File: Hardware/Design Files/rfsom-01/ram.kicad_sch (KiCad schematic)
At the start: 32 parts

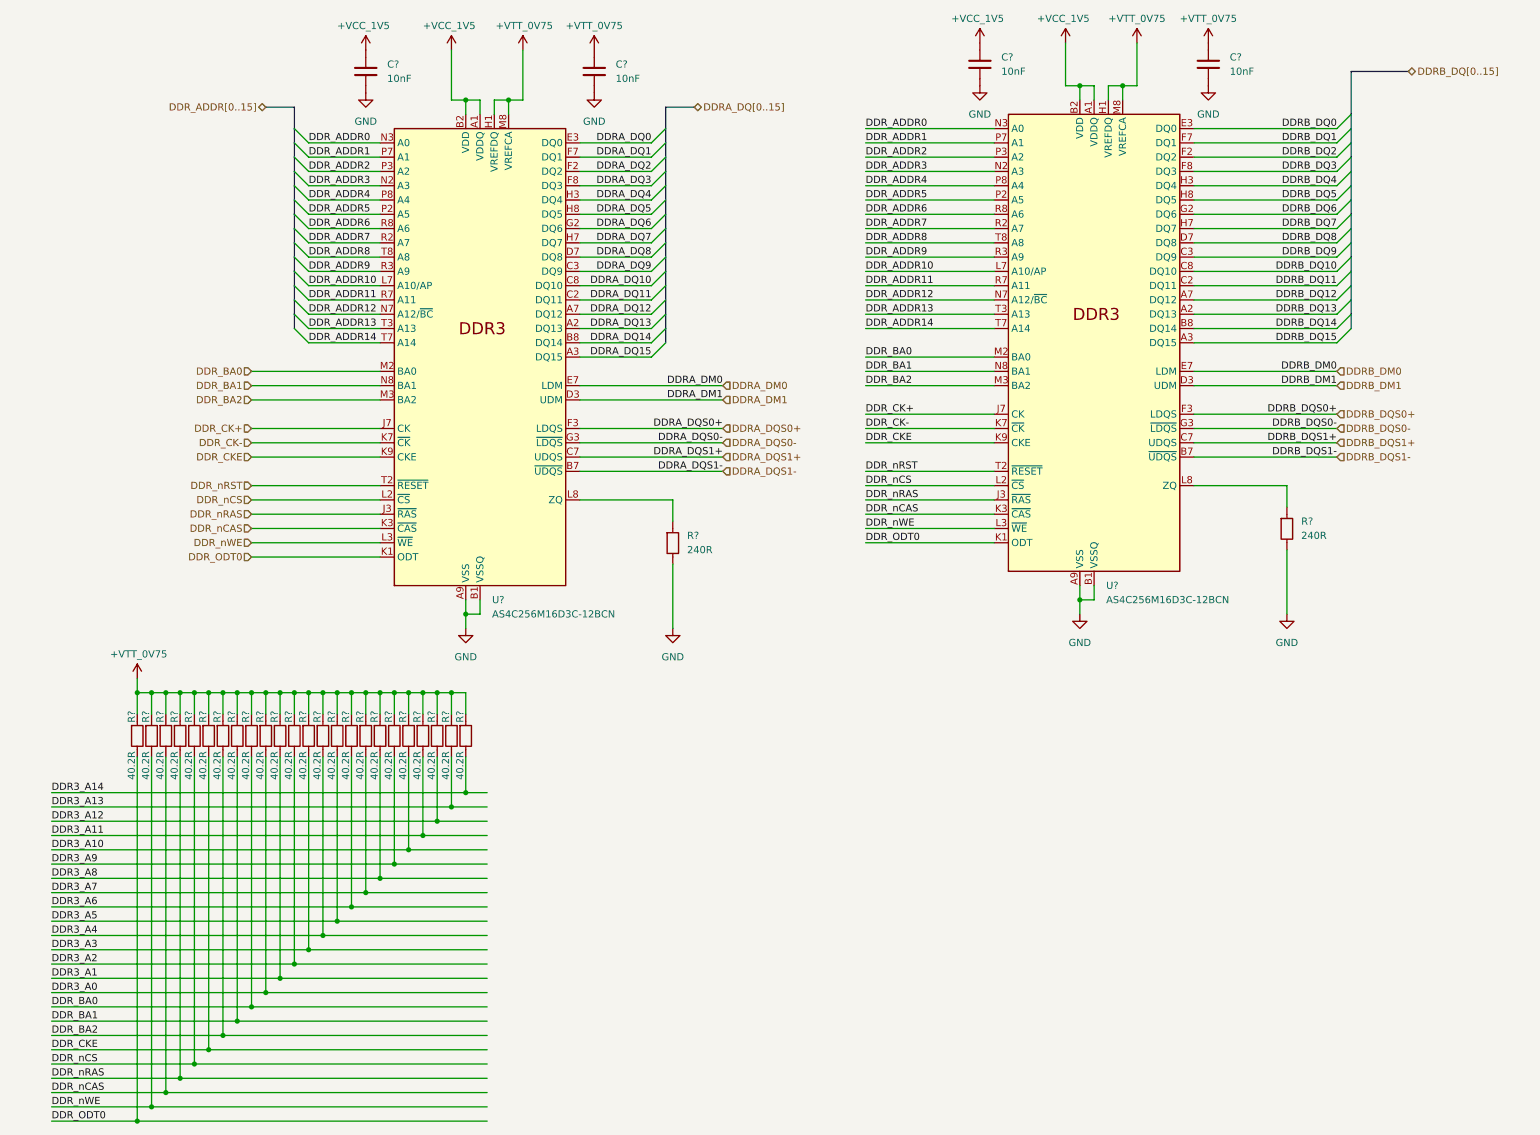
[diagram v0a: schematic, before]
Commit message: ps progress; added ftdi; mezz pinout pedinging;
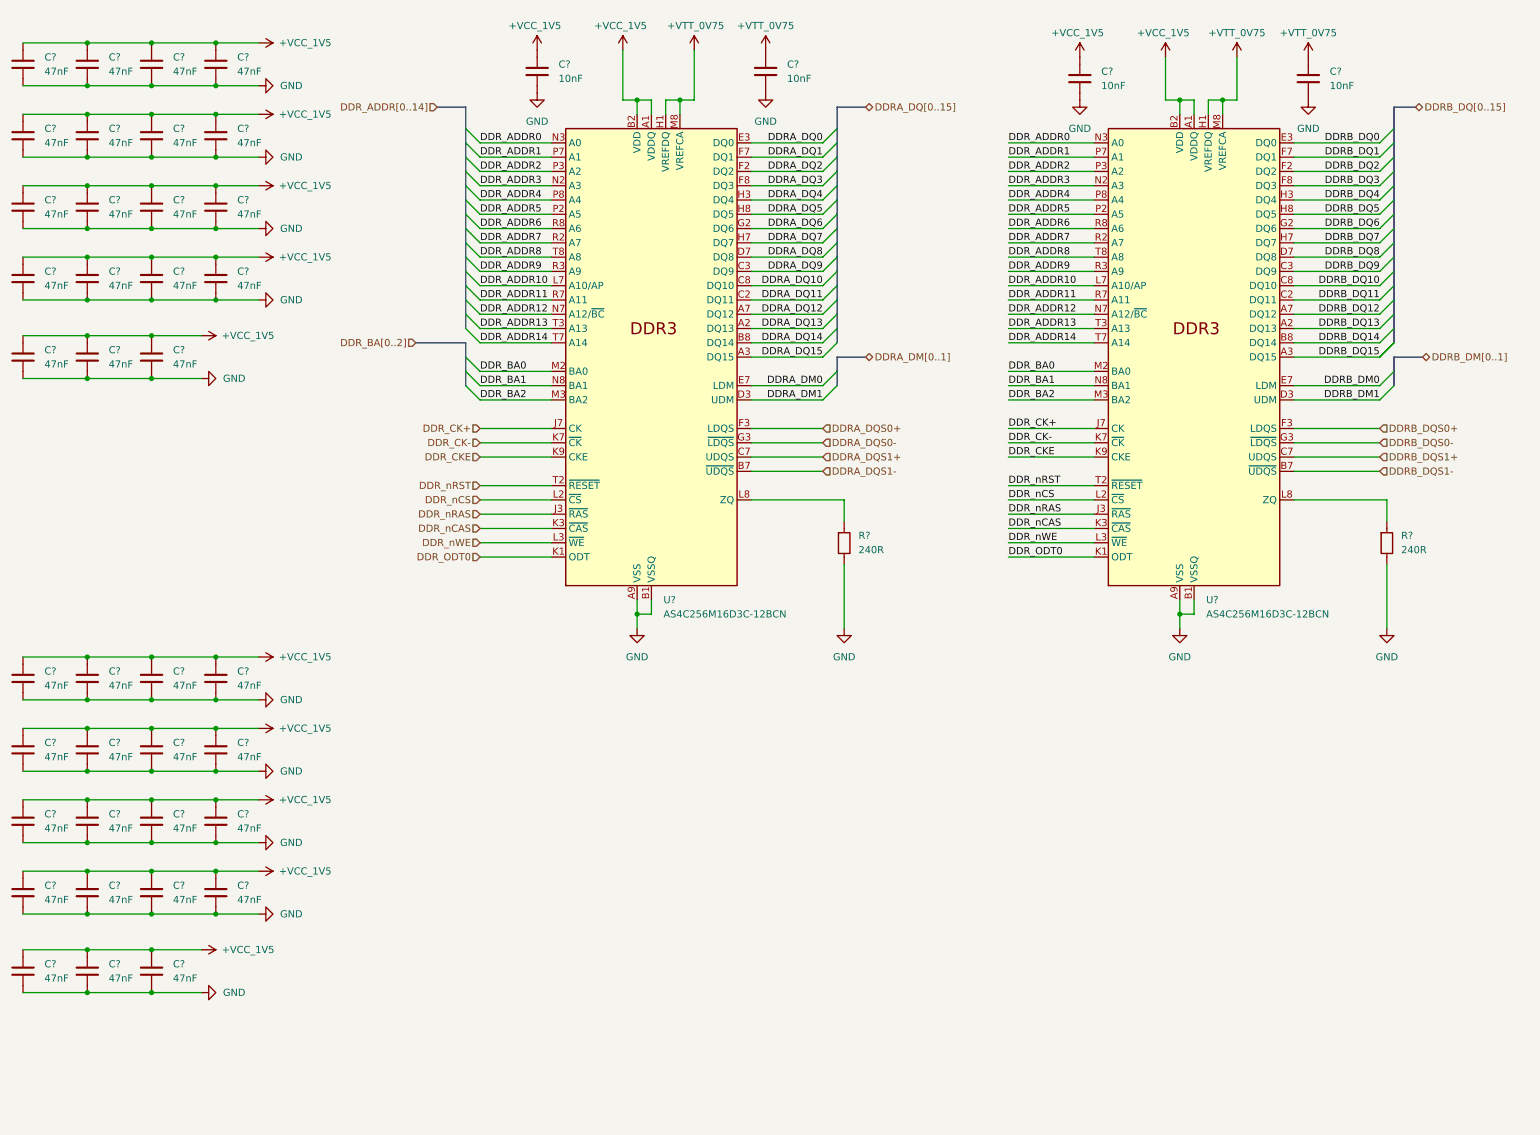
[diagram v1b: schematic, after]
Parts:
- removed R? (x24): RT0402FRE0740R2L, Resistor_SMD:R_0402_1005Metric, symbol Resistors:RT0402FRE0740R2L
- added C? (x38): CL05B473KA5VPNC, Capacitor_SMD:C_0402_1005Metric, symbol Capacitors:CL05B473KA5VPNC
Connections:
- net +VCC_1V5: now also C?.1, C?.1, C?.1, C?.1, C?.1, C?.1, C?.1, C?.1, C?.1, C?.1, C?.1, C?.1, C?.1, C?.1, C?.1, C?.1, C?.1, C?.1, C?.1, C?.1, C?.1, C?.1, C?.1, C?.1, C?.1, C?.1, C?.1, C?.1, C?.1, C?.1, C?.1, C?.1, C?.1, C?.1, C?.1, C?.1, C?.1, C?.1
- net GND: now also C?.2, C?.2, C?.2, C?.2, C?.2, C?.2, C?.2, C?.2, C?.2, C?.2, C?.2, C?.2, C?.2, C?.2, C?.2, C?.2, C?.2, C?.2, C?.2, C?.2, C?.2, C?.2, C?.2, C?.2, C?.2, C?.2, C?.2, C?.2, C?.2, C?.2, C?.2, C?.2, C?.2, C?.2, C?.2, C?.2, C?.2, C?.2
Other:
- moved on the sheet: C?, R?, U?
